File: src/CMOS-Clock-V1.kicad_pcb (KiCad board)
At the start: 4 copper layers, 100 x 61 mm, 102 parts, among them J1 USB_B_Micro, SW1 SW_Push, SW2 SW_Push, SW3 SW_Push, U1 BAS28,215, U10 74AHC86D,118, U11 74HC390D,652, U12 74HC390D,652, U13 2N7002PS, U14 MC14511BDR2G, U15 2N7002PS, U16 74LVC1G74DP,125, U17 MC14511BDR2G, U18 2N7002PS, U19 MC14511BDR2G, U2 7555, U20 2N7002PS, U21 MC14511BDR2G, U3 74AHC1G4215, U4 74AHC3G14DP,125, U5 74HC390D,652, U6 74AHC157D,118, U7 74HC27D,653, U8 74LVC1G157, U9 74AHC08D,118, X1 OM-7604-C7

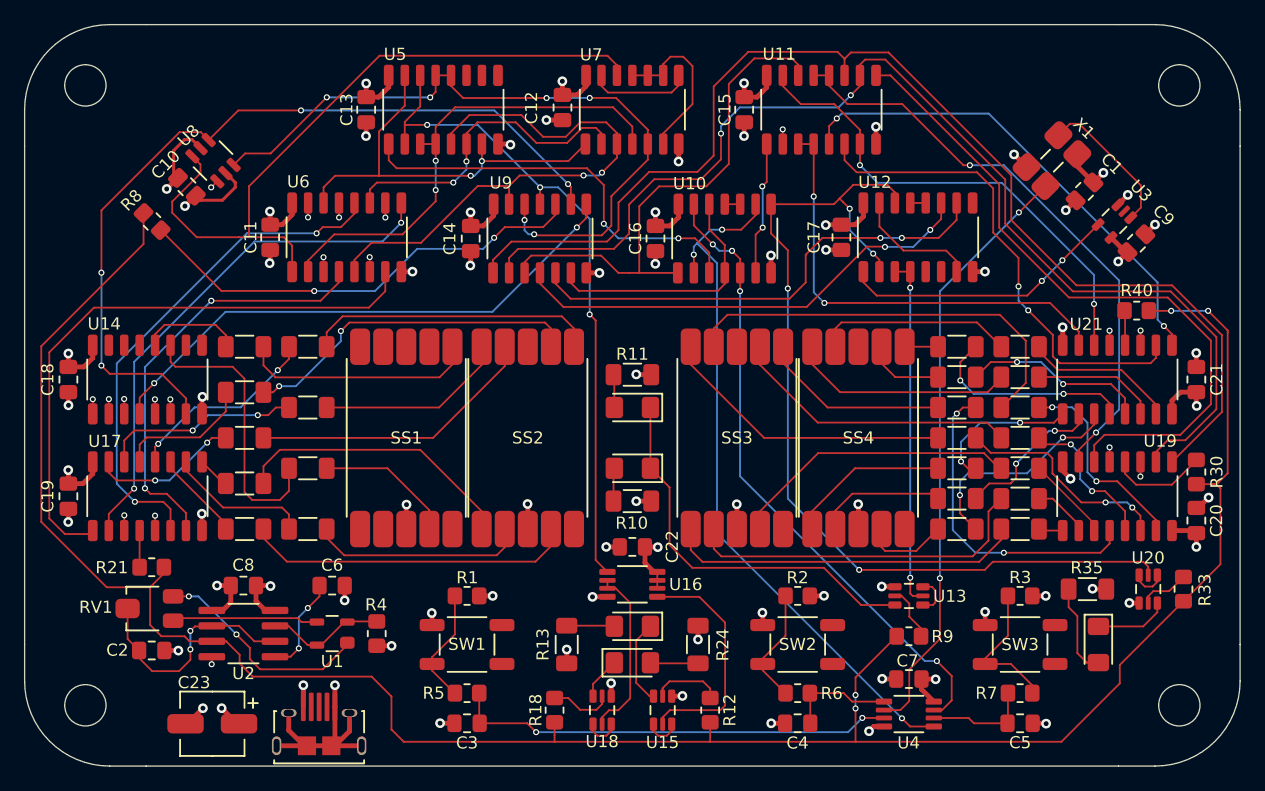
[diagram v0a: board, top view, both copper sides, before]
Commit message: Update
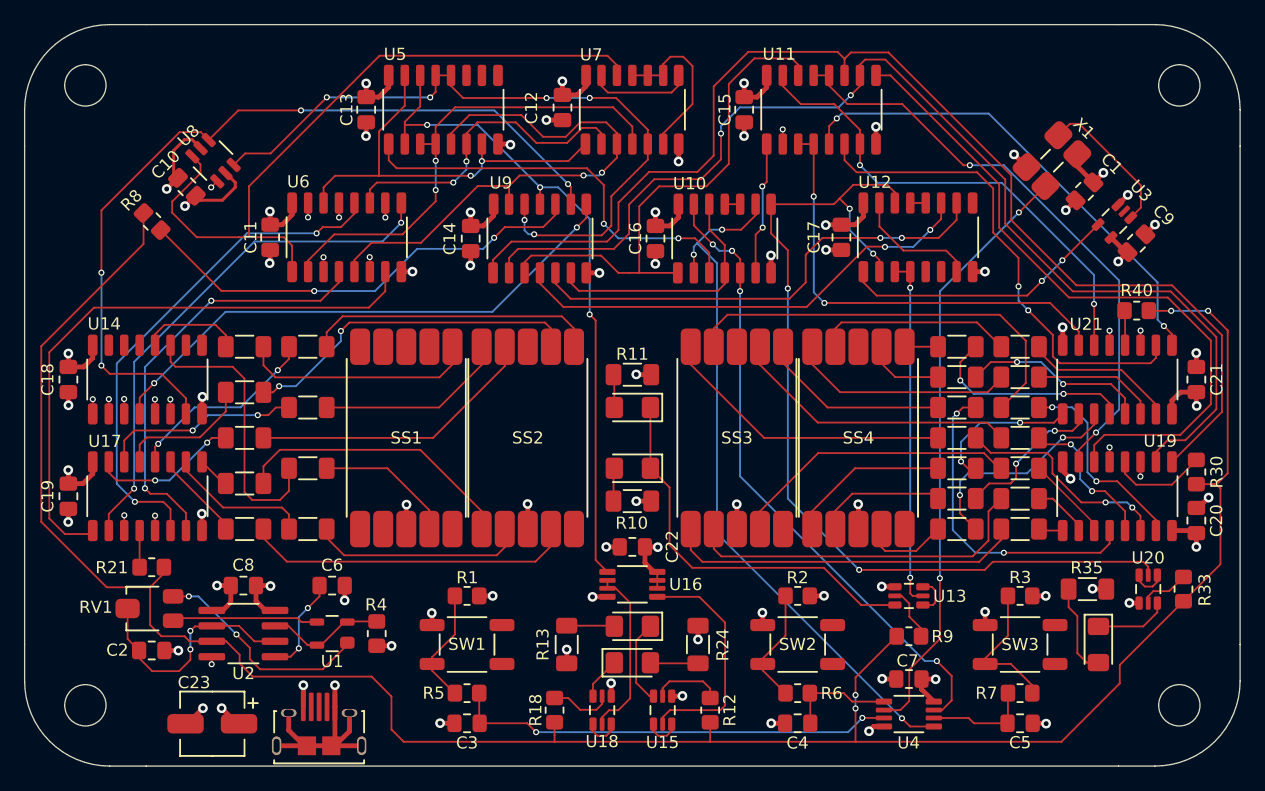
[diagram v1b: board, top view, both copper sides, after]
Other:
- net class Default removed
